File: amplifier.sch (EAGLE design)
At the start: 120 parts, among them J8 47R, Q1 2N2222, Q2 2N2222, Q3 2N2222, Q4 2N2222, Q5 2N2222, Q6 2N2222, Q7 2N2222, Q8 2N2222, T1 2N2222

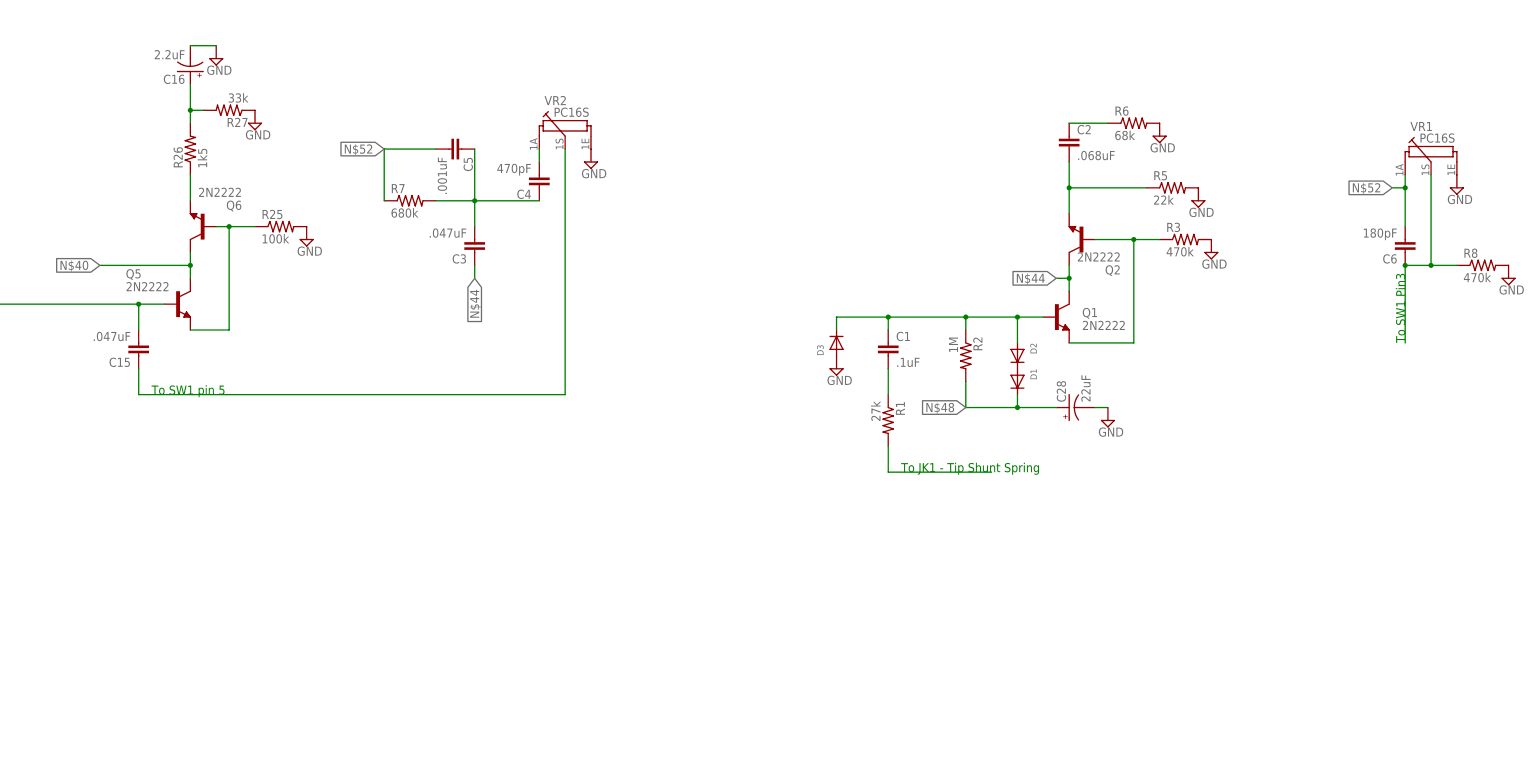
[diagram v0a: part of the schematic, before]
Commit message: cleaner clean_version
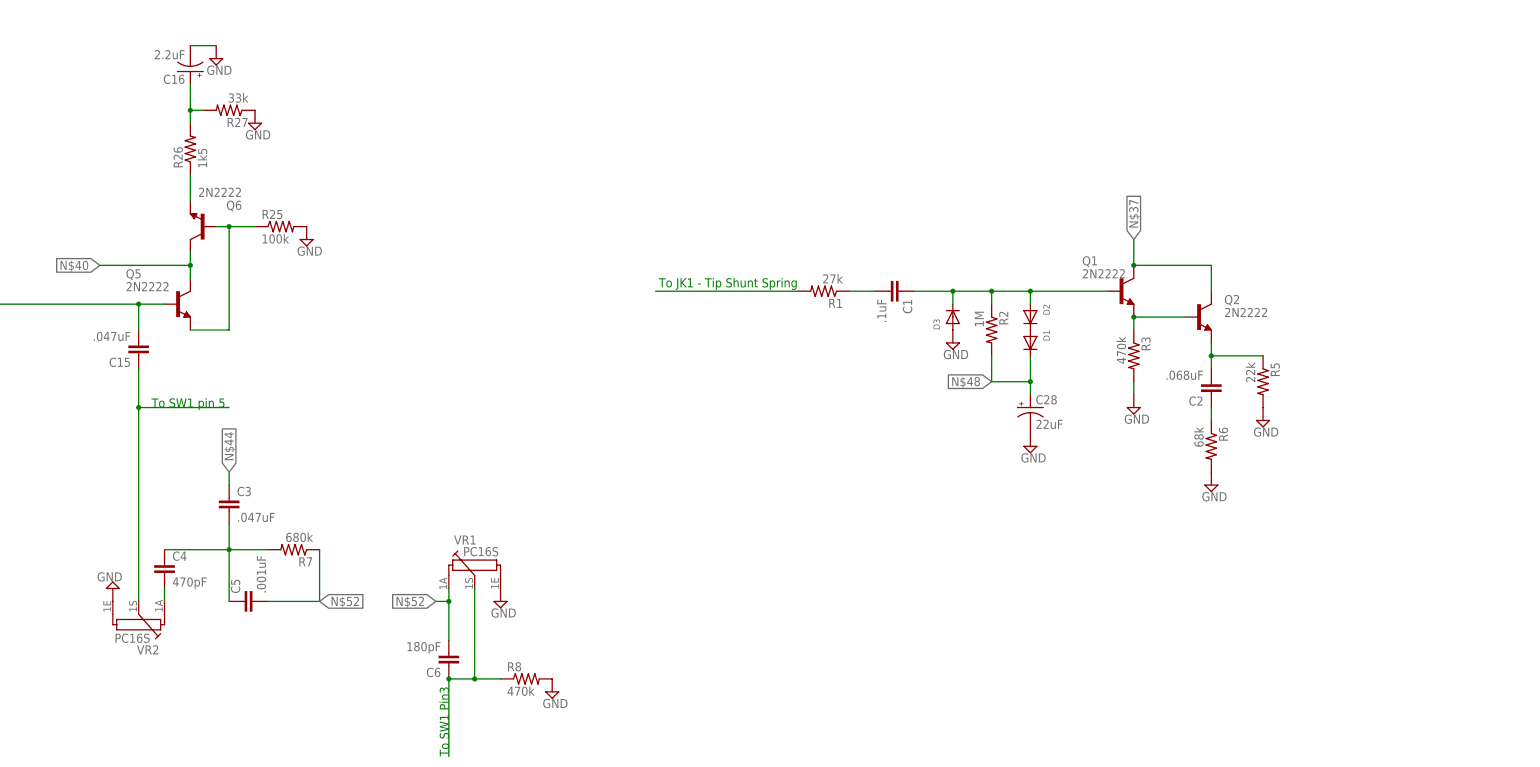
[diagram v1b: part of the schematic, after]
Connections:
- new net N$37: Q1.C, Q2.C
- net N$44: no longer Q1.C, Q2.C
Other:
- moved on the sheet: C1, C2, C28, C3, C4, C5, C6, D1, D2, D3, Q1, Q2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
